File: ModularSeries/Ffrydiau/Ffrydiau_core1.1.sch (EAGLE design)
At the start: 37 parts

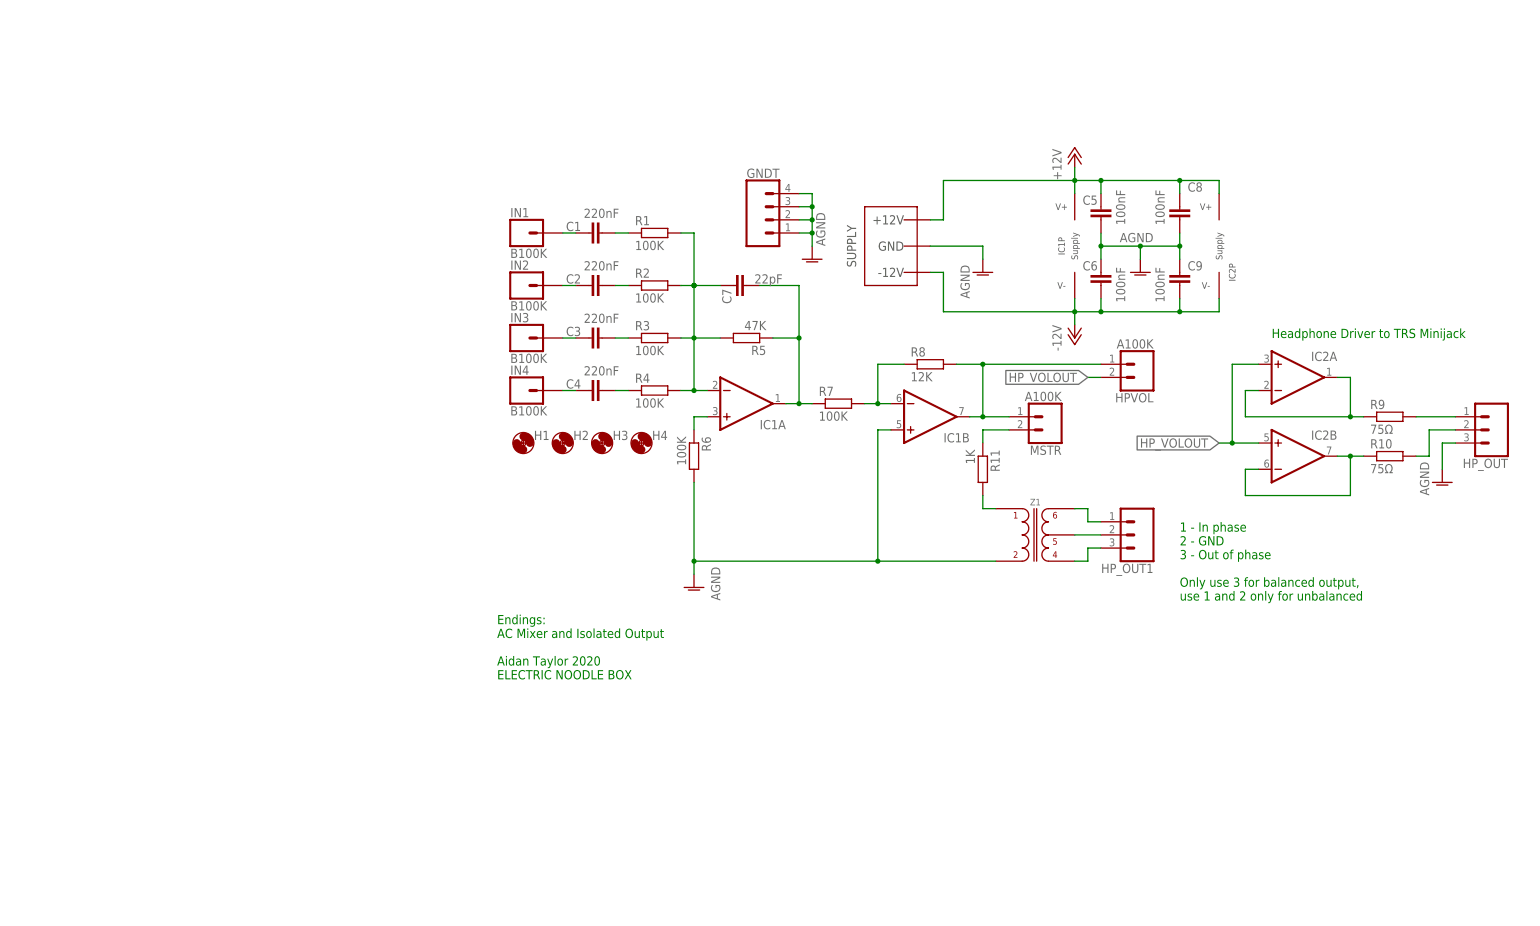
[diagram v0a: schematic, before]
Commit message: Fields added and various updates to designs
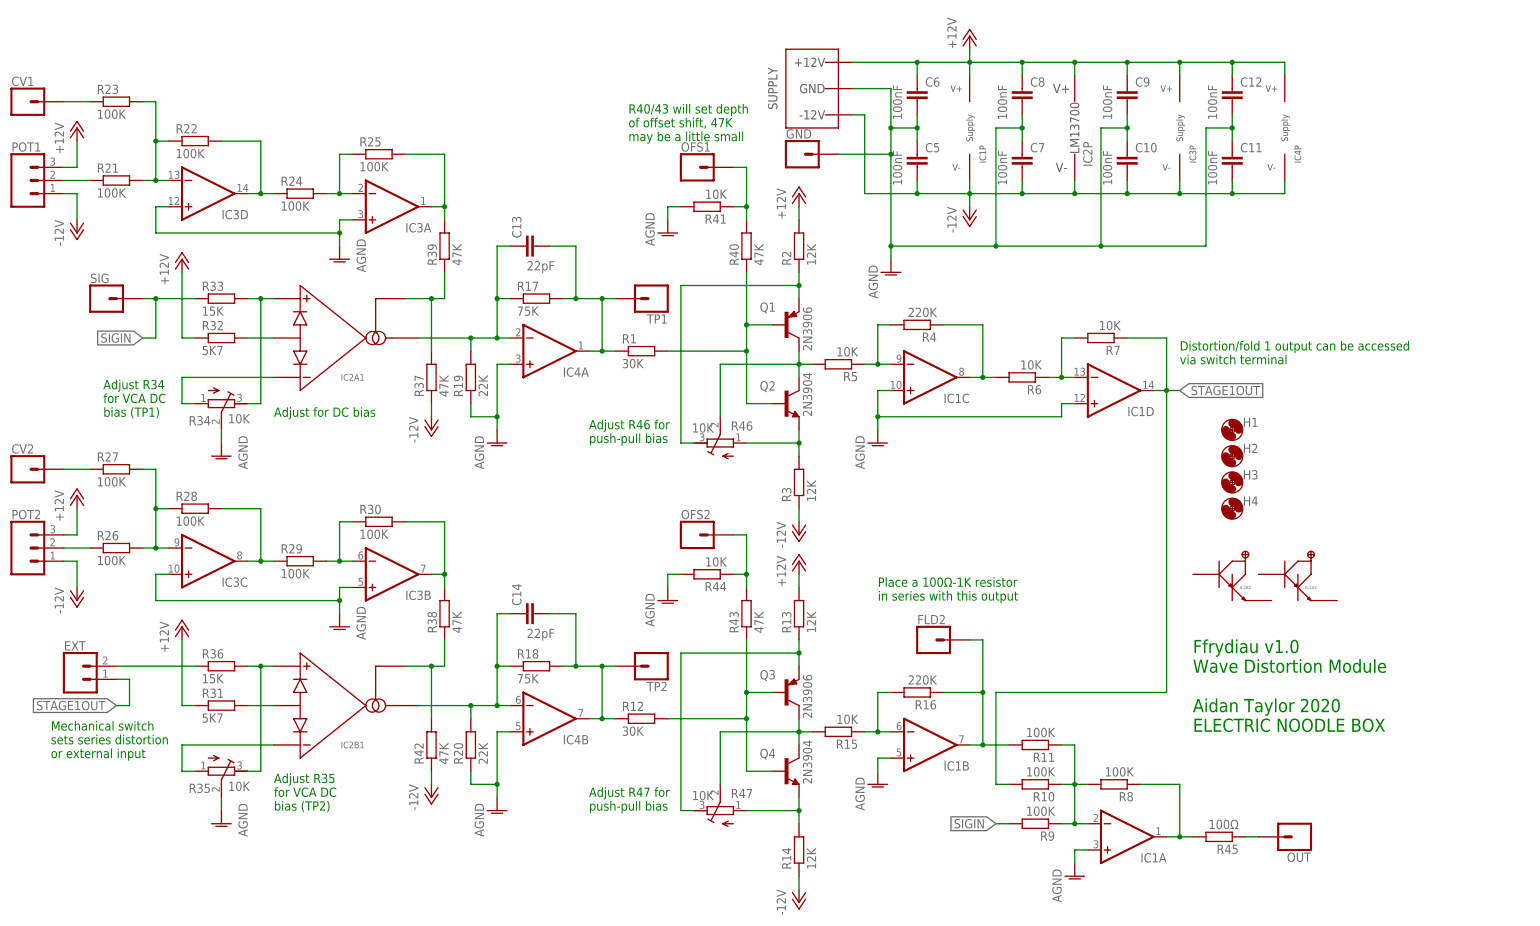
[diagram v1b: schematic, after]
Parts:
- removed C1, C2, C3, C4: 220nF, rcl:C-EU050-025X075
- removed GNDT: 4XWIREPAD, ElectricNoodleBox:4XWIREPAD
- removed HPVOL, MSTR: A100K, ElectricNoodleBox:2XWIREPAD
- removed HP_OUT, HP_OUT1: 3XWIREPAD, ElectricNoodleBox:3XWIREPAD
- removed IN1, IN2, IN3, IN4: B100K, ElectricNoodleBox:1XWIREPAD
- removed Z1: (no value), ElectricNoodleBox:Z1604_AUDIO_TRANSFORMER
- added C10, C11, C12: 100nF, rcl:C-EU050-025X075
- added C13, C14: 22pF, rcl:C-EU050-025X075
- added CV1, CV2, FLD2, GND, OFS1, OFS2, OUT, SIG, TP1, TP2: 1XWIREPAD, ElectricNoodleBox:1XWIREPAD
- added EXT: 2XWIREPAD, ElectricNoodleBox:2XWIREPAD
- added IC3: (no value), ElectricNoodleBox:TL0X4DIL
- added IC4: (no value), ElectricNoodleBox:TL0X2DIL
- added POT1, POT2: 3XWIREPAD, ElectricNoodleBox:3XWIREPAD
- added Q1, Q3: 2N3906, transistor-pnp:2N3906
- added Q2, Q4: 2N3904, transistor-npn:2N3904
- added R12: 30K, rcl:R-EU_0207/7
- added R13, R14: 12K, rcl:R-EU_0207/7
- added R15, R41, R44: 10K, rcl:R-EU_0207/7
- added R16: 220K, rcl:R-EU_0207/7
- added R17, R18: 75K, rcl:R-EU_0207/7
- added R19, R20: 22K, rcl:R-EU_0207/7
- added R21, R22, R23, R24, R25, R26, R27, R28, R29, R30: 100K, rcl:R-EU_0207/7
- added R31, R32: 5K7, rcl:R-EU_0207/7
- added R33, R36: 15K, rcl:R-EU_0207/7
- added R34, R35, R46, R47: 10K, rcl:R-TRIMM3296W
- added R37, R38, R39, R40, R42, R43: 47K, rcl:R-EU_0207/7
- added R45: 100Ω, rcl:R-EU_0207/7
- C7: value 22pF -> 100nF
- IC1: device ElectricNoodleBox:TL0X2DIL -> ElectricNoodleBox:TL0X4DIL
- IC2: device ElectricNoodleBox:TL0X2DIL -> ElectricNoodleBox:LM13700DIL
- R1: value 100K -> 30K; device rcl:R-EU_0207/10 -> rcl:R-EU_0207/7
- R10, R9: value 75Ω -> 100K; device rcl:R-EU_0207/10 -> rcl:R-EU_0207/7
- R11: value 1K -> 100K; device rcl:R-EU_0207/10 -> rcl:R-EU_0207/7
- R2, R3: value 100K -> 12K; device rcl:R-EU_0207/10 -> rcl:R-EU_0207/7
- R4: value 100K -> 220K; device rcl:R-EU_0207/10 -> rcl:R-EU_0207/7
- R5: value 47K -> 10K; device rcl:R-EU_0207/10 -> rcl:R-EU_0207/7
- R6, R7: value 100K -> 10K; device rcl:R-EU_0207/10 -> rcl:R-EU_0207/7
- R8: value 12K -> 100K; device rcl:R-EU_0207/10 -> rcl:R-EU_0207/7
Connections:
- removed net HP_VOLOUT: HPVOL.2, IC2A.+IN, IC2B.+IN
- removed net N$10: C3.2, R3.1
- removed net N$11: C4.2, R4.1
- removed net N$12: C2.1, IN2.1
- new net N$23: C14.2, IC4B.OUT, R12.1, R18.2, TP2.1
- new net N$24: IC3D.-IN, R21.2, R22.1, R23.2
- new net N$25: IC3D.OUT, R22.2, R24.1
- new net N$26: IC3A.-IN, R24.2, R25.1
- new net N$27: IC3A.OUT, R25.2, R39.2
- new net N$28: CV2.1, R27.1
- new net N$29: IC3B.OUT, R30.2, R38.2
- new net N$30: POT1.2, R21.1
- new net N$31: IC3B.-IN, R29.2, R30.1
- new net N$32: CV1.1, R23.1
- new net N$33: IC3C.OUT, R28.2, R29.1
- new net N$34: IC3C.-IN, R26.2, R27.2, R28.1
- new net N$35: IC2B1.AMP+, R35.E, R36.2
- new net N$36: IC2B1.AMP-, R35.A
- new net N$37: IC2B1.DIODES, R31.2
- new net N$38: IC2A1.DIODES, R32.2
- new net N$39: IC2A1.AMPBIAS, R37.2, R39.1
- new net N$40: POT2.2, R26.1
- new net N$41: IC2A1.AMP+, R33.2, R34.E
- new net N$42: IC2A1.AMP-, R34.A
- new net N$43: IC2B1.AMPBIAS, R38.1, R42.2
- new net N$44: OFS1.1, R40.2, R41.1
- new net N$45: OFS2.1, R43.2, R44.1
- new net N$47: EXT.2, R36.1
- new net SIGIN: R33.1, R9.2, SIG.1
- new net STAGE1OUT: EXT.1, IC1D.OUT, R10.2, R7.1
- net +12V: now also C12.1, C6.1, C9.1, IC3P.V+, IC4P.V+, POT1.3, POT2.3, R13.2, R2.2, R31.1, R32.1; no longer C5.1
- net -12V: now also C10.2, C11.2, C5.2, C7.2, IC3P.V-, IC4P.V-, POT1.1, POT2.1, R14.1, R3.1, R37.1, R42.1; no longer C6.2, C9.2
- net AGND: now also C10.1, C11.1, C12.2, C5.1, C6.2, C7.1, C9.2, GND.1, IC1A.+IN, IC1C.+IN, IC1D.+IN, IC3A.+IN, IC3B.+IN, IC3C.+IN, IC3D.+IN, IC4A.+IN, IC4B.+IN, R19.1, R20.1, R34.S, R35.S, R41.2, R44.2; no longer C5.2, C6.1, C9.1, GNDT.1, GNDT.2, GNDT.3, GNDT.4, HP_OUT.3, R6.2, Z1.3
- net N$1: now also Q1.B, Q2.B, R1.2, R40.1; no longer C4.1, IN4.1
- net N$13: now also IC1A.-IN, R10.1, R11.1, R8.2, R9.1; no longer C1.1, IN1.1
- net N$14: now also IC1A.OUT, R45.2, R8.1; no longer MSTR.2, R11.1
- net N$15: now also Q3.B, Q4.B, R12.2, R43.1; no longer HP_OUT1.1, Z1.6
- net N$16: now also Q3.E, R13.1, R47.E; no longer HP_OUT1.2, Z1.5
- net N$17: now also Q4.E, R14.2, R47.A; no longer HP_OUT1.3, Z1.4
- net N$18: now also Q3.C, Q4.C, R15.2, R47.S; no longer IC2A.-IN, IC2A.OUT, R9.1
- net N$19: now also IC1B.-IN, R15.1, R16.2; no longer HP_OUT.1, R9.2
- net N$2: now also Q1.E, R2.1, R46.E; no longer C7.1, IC1A.-IN, R1.2, R2.2, R3.2, R4.2, R5.2
- net N$20: now also FLD2.1, IC1B.OUT, R11.2, R16.1; no longer IC2B.-IN, IC2B.OUT, R10.1
- net N$21: now also C14.1, IC2B1.AMPOUT, IC4B.-IN, R18.1, R20.2; no longer HP_OUT.2, R10.2
- net N$22: now also C13.1, IC2A1.AMPOUT, IC4A.-IN, R17.1, R19.2; no longer R11.2, Z1.1
- net N$3: now also Q2.E, R3.2, R46.A; no longer C7.2, IC1A.OUT, R5.1, R7.1
- net N$4: now also Q1.C, Q2.C, R46.S, R5.2; no longer IC1B.-IN, R7.2, R8.1
- net N$5: now also IC1C.-IN, R4.2, R5.1; no longer HPVOL.1, IC1B.OUT, MSTR.1, R8.2
- net N$6: now also IC1C.OUT, R4.1, R6.2; no longer C3.1, IN3.1
- net N$7: now also IC1D.-IN, R7.2; no longer IC1A.+IN
- net N$8: now also OUT.1, R45.1; no longer C1.2, R1.1
- net N$9: now also C13.2, IC4A.OUT, R1.1, R17.2, TP1.1; no longer C2.2, R2.1
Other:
- note added: "Adjust R34 for VCA DC bias (TP1)"
- note added: "Adjust R35 for VCA DC bias (TP2)"
- note added: "Adjust R46 for push-pull bias"
- note added: "Adjust R47 for push-pull bias"
- note added: "Adjust for DC bias"
- note added: "Distortion/fold 1 output can be accessed via switch terminal"
- note added: "Ffrydiau v1.0 Wave Distortion Module Aidan Taylor 2020 ELECTRIC NOODLE BOX"
- note added: "Mechanical switch sets series distortion or external input"
- note added: "Place a 100Ω-1K resistor in series with this output"
- note added: "R40/43 will set depth of offset shift, 47K may be a little small"
- note removed: "1 - In phase 2 - GND 3 - Out of phase Only use 3 for balanced output, use 1 and 2 only for unbalanced"
- note removed: "Endings: AC Mixer and Isolated Output Aidan Taylor 2020 ELECTRIC NOODLE BOX"
- note removed: "Headphone Driver to TRS Minijack"
- moved on the sheet: C5, C6, C7, C8, C9, H1, H2, H3, H4, IC1A, IC1B, IC1P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
